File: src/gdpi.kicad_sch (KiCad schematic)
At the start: 24 parts, among them J7 HDMI_C_1.3, U1 ECP5U_12_CABGA256, U9 PCA9306DC1, Y1 ECS-2520MV-xxx-xx

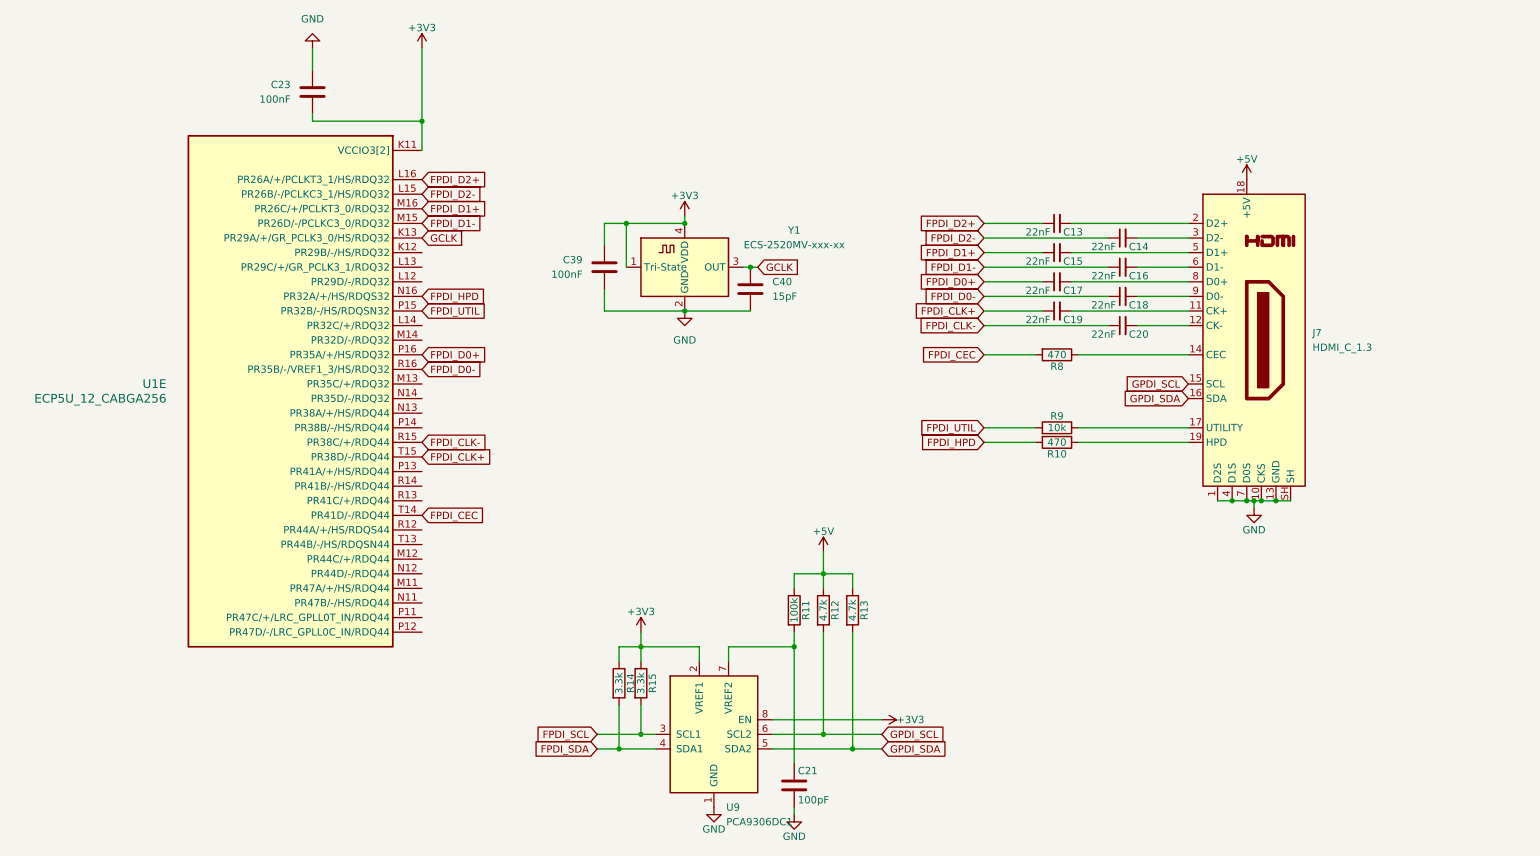
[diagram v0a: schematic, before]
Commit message: Rev 2
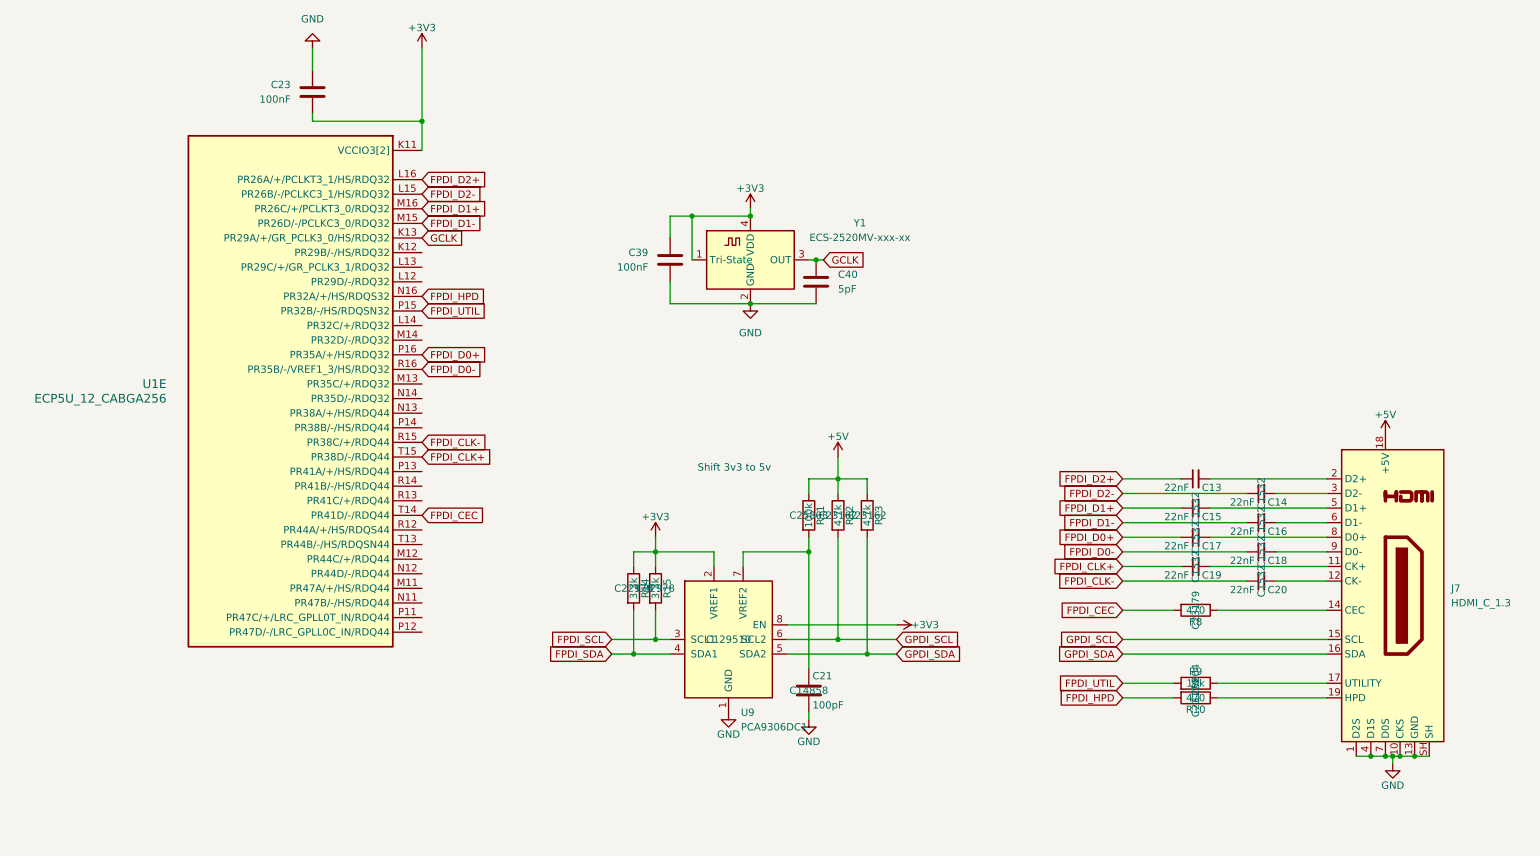
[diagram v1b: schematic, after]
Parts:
- C13, C14, C15, C16, C17, C18, C19, C20: footprint Capacitor_SMD:C_0603_1608Metric -> Capacitor_SMD:C_0402_1005Metric; LCSC Part (none) -> C1532
- C21: LCSC Part (none) -> C14858
- C23, C39: LCSC Part (none) -> C1525
- C40: value 15pF -> 5pF; LCSC Part (none) -> C541339
- R10, R8: LCSC Part (none) -> C23179
- R11: LCSC Part (none) -> C25803
- R12, R13: LCSC Part (none) -> C23162
- R14, R15: LCSC Part (none) -> C22978
- R9: LCSC Part (none) -> C25804
- U9: LCSC Part (none) -> C129510
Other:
- note added: "Shift 3v3 to 5v"
- moved on the sheet: C13, C14, C15, C16, C17, C18, C19, C20, C21, C39, C40, J7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

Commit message: Tidy project
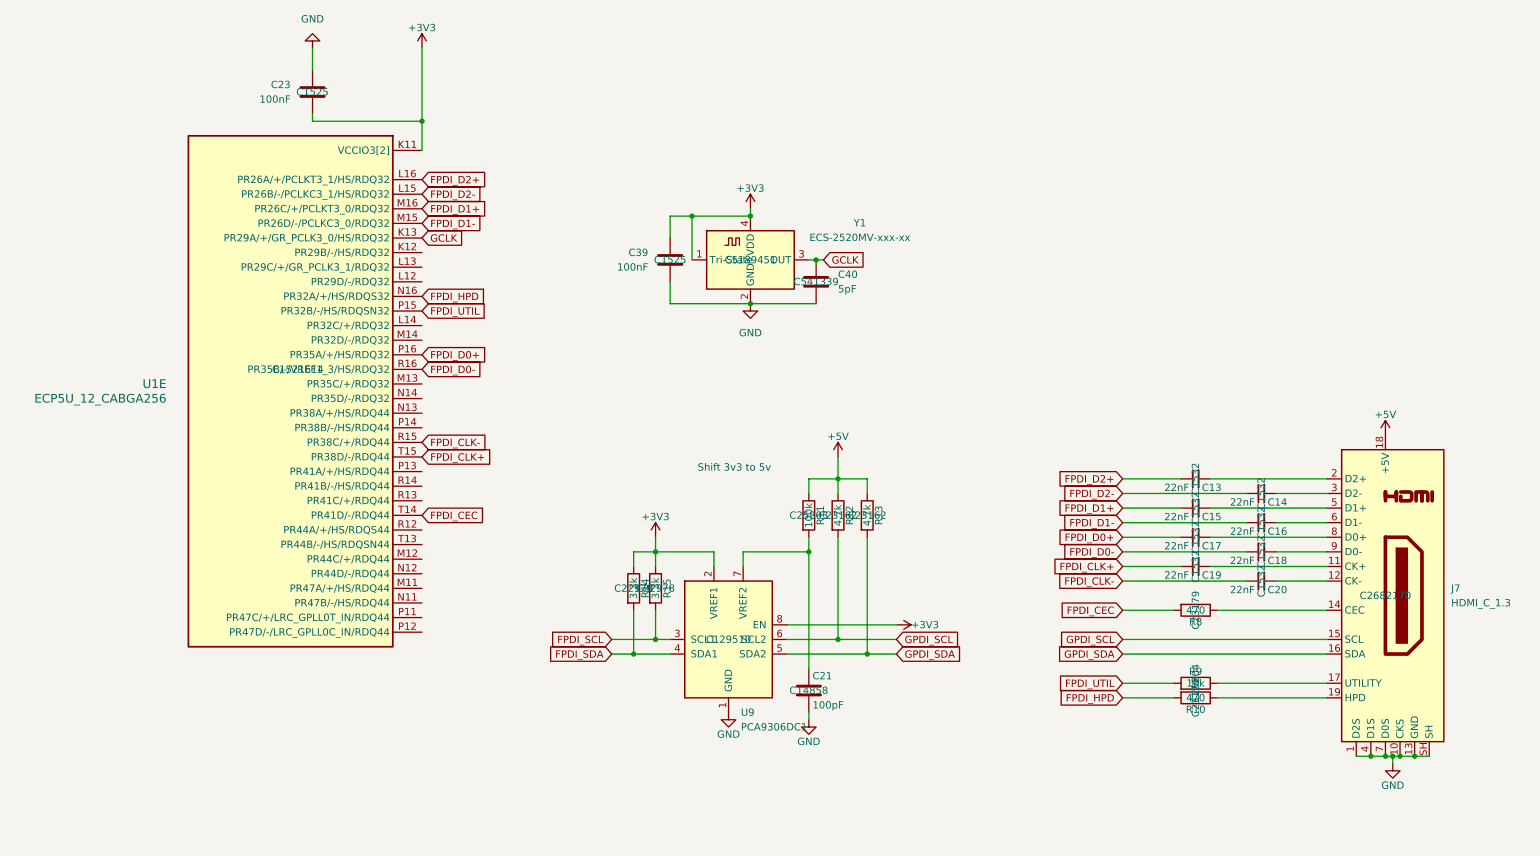
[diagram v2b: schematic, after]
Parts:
- C13, C14, C15, C16, C17, C18, C19, C20: JLCPCB Part # (none) -> C1532; LCSC Part C1532 -> (none)
- C21: JLCPCB Part # (none) -> C14858; LCSC Part C14858 -> (none)
- C23, C39: JLCPCB Part # (none) -> C1525; LCSC Part C1525 -> (none)
- C40: JLCPCB Part # (none) -> C541339; LCSC Part C541339 -> (none)
- J7: JLCPCB Part # (none) -> C2682170; LCSC Part C2682170 -> (none)
- R10, R8: JLCPCB Part # (none) -> C23179; LCSC Part C23179 -> (none)
- R11: JLCPCB Part # (none) -> C25803; LCSC Part C25803 -> (none)
- R12, R13: JLCPCB Part # (none) -> C23162; LCSC Part C23162 -> (none)
- R14, R15: JLCPCB Part # (none) -> C22978; LCSC Part C22978 -> (none)
- R9: JLCPCB Part # (none) -> C25804; LCSC Part C25804 -> (none)
- U1: JLCPCB Part # (none) -> C1521614; LCSC Part C1521614 -> (none)
- U9: JLCPCB Part # (none) -> C129510; LCSC Part C129510 -> (none)
- Y1: JLCPCB Part # (none) -> C5189451; LCSC Part C5189451 -> (none)
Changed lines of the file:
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@@
 			)
 		)
-		(property "LCSC Part" "C25803"
+		(property "JLCPCB Part #" "C25803"
 			(at 158.75 109.22 0)
 			(effects
@@
 			)
 		)
-		(property "LCSC Part" "C23162"
+		(property "JLCPCB Part #" "C23162"
 			(at 163.83 109.22 0)
 			(effects
@@
 			)
 		)
-		(property "LCSC Part" "C23162"
+		(property "JLCPCB Part #" "C23162"
 			(at 168.91 109.22 0)
 			(effects
@@
 			)
 		)
-		(property "LCSC Part" "C14858"
+		(property "JLCPCB Part #" "C14858"
 			(at 158.75 139.7 0)
 			(effects
@@
 			)
 		)
-		(property "LCSC Part" "C22978"
+		(property "JLCPCB Part #" "C22978"
 			(at 132.08 121.92 0)
 			(effects
@@
 			)
 		)
-		(property "LCSC Part" "C22978"
+		(property "JLCPCB Part #" "C22978"
 			(at 128.27 121.92 0)
 			(effects
@@
 			)
 		)
-		(property "LCSC Part" "C23179"
+		(property "JLCPCB Part #" "C23179"
 			(at 226.06 140.97 0)
 			(effects
@@
 			)
 		)
-		(property "LCSC Part" "C2682170 "
+		(property "JLCPCB Part #" "C2682170 "
 			(at 259.08 123.19 0)
 			(effects
@@
 					(size 1.27 1.27)
 				)
-				(hide yes)
 			)
 		)
@@
 			)
 		)
-		(property "LCSC Part" "C1532"
+		(property "JLCPCB Part #" "C1532"
 			(at 226.06 107.95 0)
 			(effects
@@
 			)
 		)
-		(property "LCSC Part" "C1532"
+		(property "JLCPCB Part #" "C1532"
 			(at 237.49 120.65 0)
 			(effects
@@
 			)
 		)
-		(property "LCSC Part" "C1532"
+		(property "JLCPCB Part #" "C1532"
 			(at 237.49 115.57 0)
 			(effects
@@
 			)
 		)
-		(property "LCSC Part" "C1525"
+		(property "JLCPCB Part #" "C1525"
 			(at 72.39 35.56 0)
 			(effects
@@
 					(size 1.27 1.27)
 				)
-				(hide yes)
 			)
 		)
@@
 			)
 		)
-		(property "LCSC Part" "C1532"
+		(property "JLCPCB Part #" "C1532"
 			(at 226.06 113.03 0)
 			(effects
@@
 			)
 		)
-		(property "LCSC Part" "C1532"
+		(property "JLCPCB Part #" "C1532"
 			(at 226.06 102.87 0)
 			(effects
@@
 					(size 1.27 1.27)
 				)
-				(hide yes)
 			)
 		)
@@
 			)
 		)
-		(property "LCSC Part" "C23179"
+		(property "JLCPCB Part #" "C23179"
 			(at 226.06 125.73 0)
 			(effects
@@
 			)
 		)
-		(property "LCSC Part" " C1521614"
+		(property "JLCPCB Part #" " C1521614"
 			(at 69.85 83.82 0)
 			(effects
@@
 					(size 1.27 1.27)
 				)
-				(hide yes)
 			)
 		)
@@
 			)
 		)
-		(property "LCSC Part" "C1532"
+		(property "JLCPCB Part #" "C1532"
 			(at 226.06 118.11 0)
 			(effects
@@
 			)
 		)
-		(property "LCSC Part" "C1532"
+		(property "JLCPCB Part #" "C1532"
 			(at 237.49 110.49 0)
 			(effects
@@
 			)
 		)
-		(property "LCSC Part" "C25804"
+		(property "JLCPCB Part #" "C25804"
 			(at 226.06 138.43 0)
 			(effects
@@
 			)
 		)
-		(property "LCSC Part" " C5189451"
+		(property "JLCPCB Part #" " C5189451"
 			(at 148.59 64.77 0)
 			(effects
@@
 					(size 1.27 1.27)
 				)
-				(hide yes)
 			)
 		)
@@
 			)
 		)
-		(property "LCSC Part" "C541339"
+		(property "JLCPCB Part #" "C541339"
 			(at 160.02 68.58 0)
 			(effects
@@
 					(size 1.27 1.27)
 				)
-				(hide yes)
 			)
 		)
@@
 			)
 		)
-		(property "LCSC Part" "C129510"
+		(property "JLCPCB Part #" "C129510"
 			(at 144.78 130.81 0)
 			(effects
@@
 			)
 		)
-		(property "LCSC Part" "C1532"
+		(property "JLCPCB Part #" "C1532"
 			(at 237.49 105.41 0)
 			(effects
@@
 			)
 		)
-		(property "LCSC Part" "C1525"
+		(property "JLCPCB Part #" "C1525"
 			(at 134.62 64.77 0)
 			(effects
@@
 					(size 1.27 1.27)
 				)
-				(hide yes)
-			)
-		)
+			)
+		)
